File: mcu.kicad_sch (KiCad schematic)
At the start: 23 parts, among them J1 USB_B_Micro, J2 PRG, U1 STM32L412CBTxP, Y1 32,768KHz, Y2 16MHz

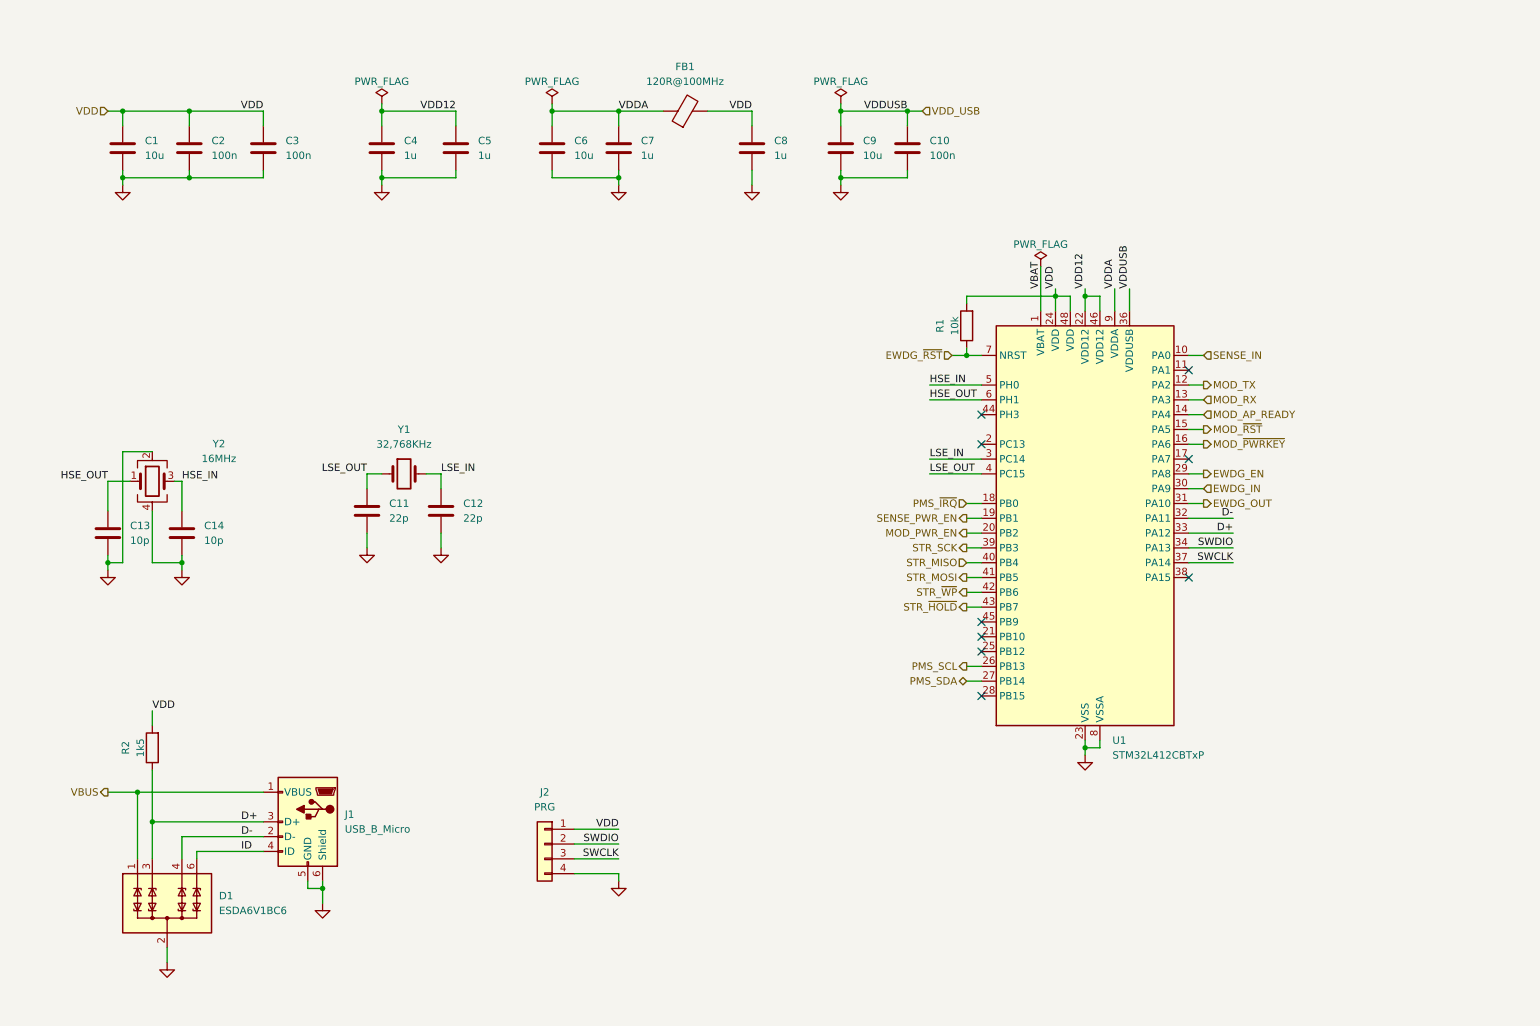
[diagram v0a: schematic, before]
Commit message: adding datasheet
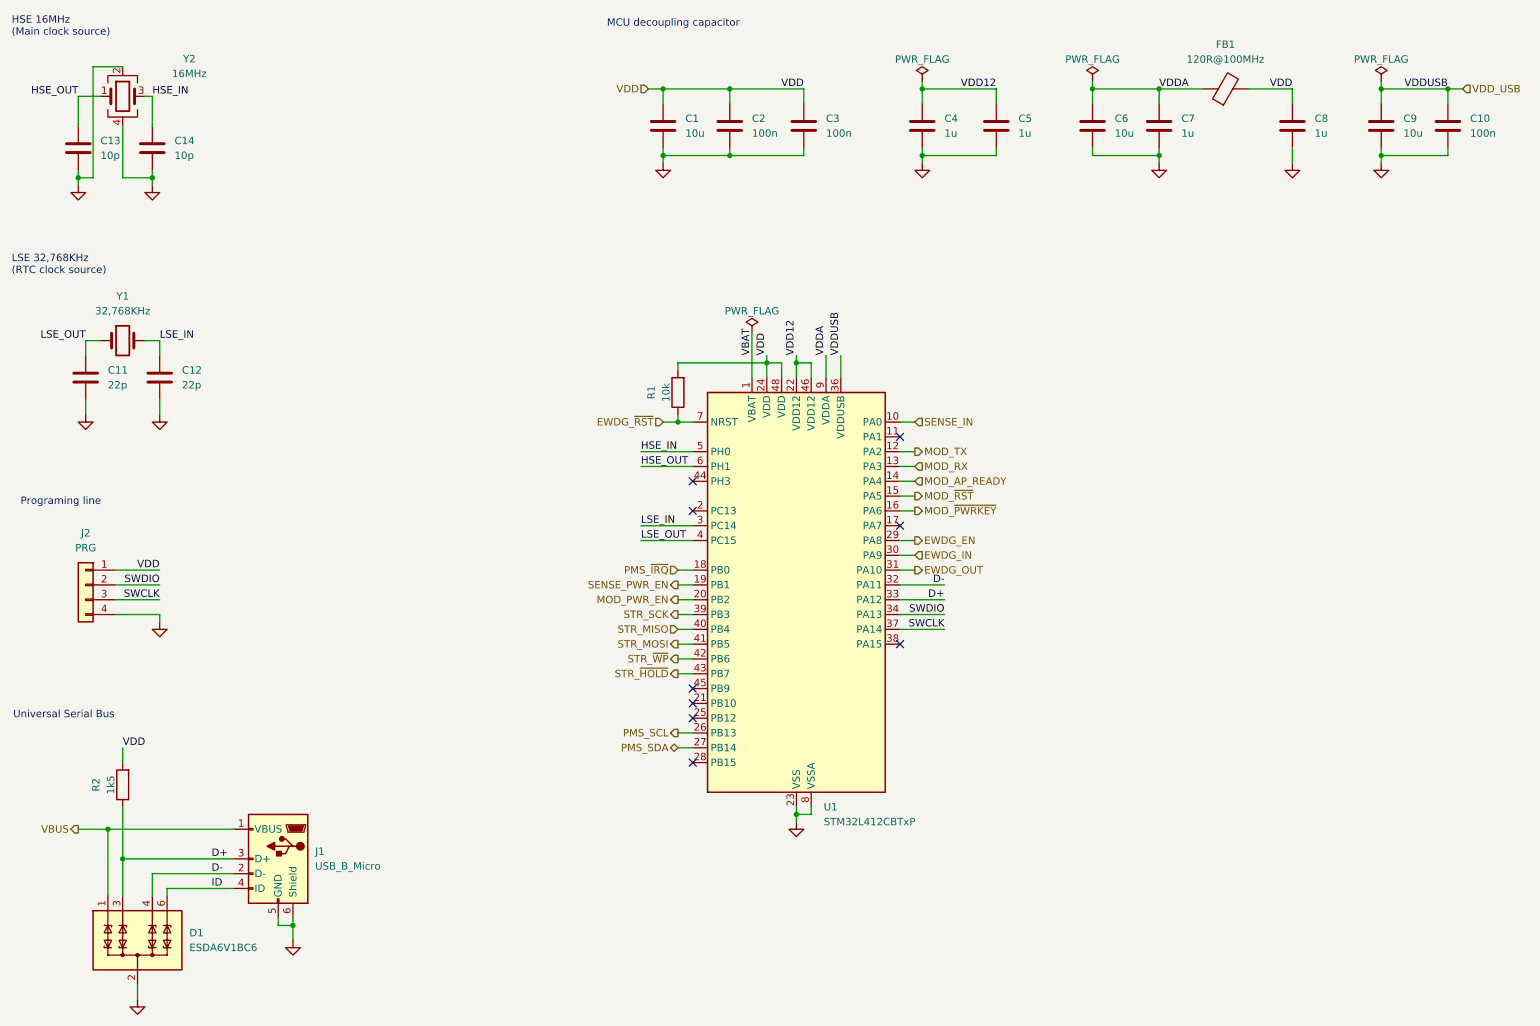
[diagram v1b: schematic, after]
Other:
- note added: "HSE 16MHz (Main clock source)"
- note added: "LSE 32,768KHz (RTC clock source)"
- note added: "MCU decoupling capacitor"
- note added: "Programing line"
- note added: "Universal Serial Bus"
- moved on the sheet: C1, C10, C11, C12, C13, C14, C2, C3, C4, C5, C6, C7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
